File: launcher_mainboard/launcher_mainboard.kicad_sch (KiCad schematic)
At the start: 76 parts, among them J10 header, J11 header, J12 USB_C_Receptacle_USB2.0_16P, J2 Conn_01x06, J3 Conn_01x06, J4 Conn_01x06, J5 Conn_01x06, J6 bat_con, J7 fan_con, J8 ESC_1, J9 ESC_2, Q1 PJC7400, Q4 BSS138, Q5 BSS138, Q6 BSS138, Q7 BSS138, SW1 POWER_SWITCH, U1 R-78E3.3-1.0, U10 TLV75533PDBV, U12 LM66200DRLR, U2 TMC2209-LA-T, U3 TMC2209-LA-T, U4 TMC2209-LA-T, U5 TMC2209-LA-T, U6 ESP32-S3-WROOM-1, U8 D3V3XA4B10LP, U9 R-78E5.0-0.5

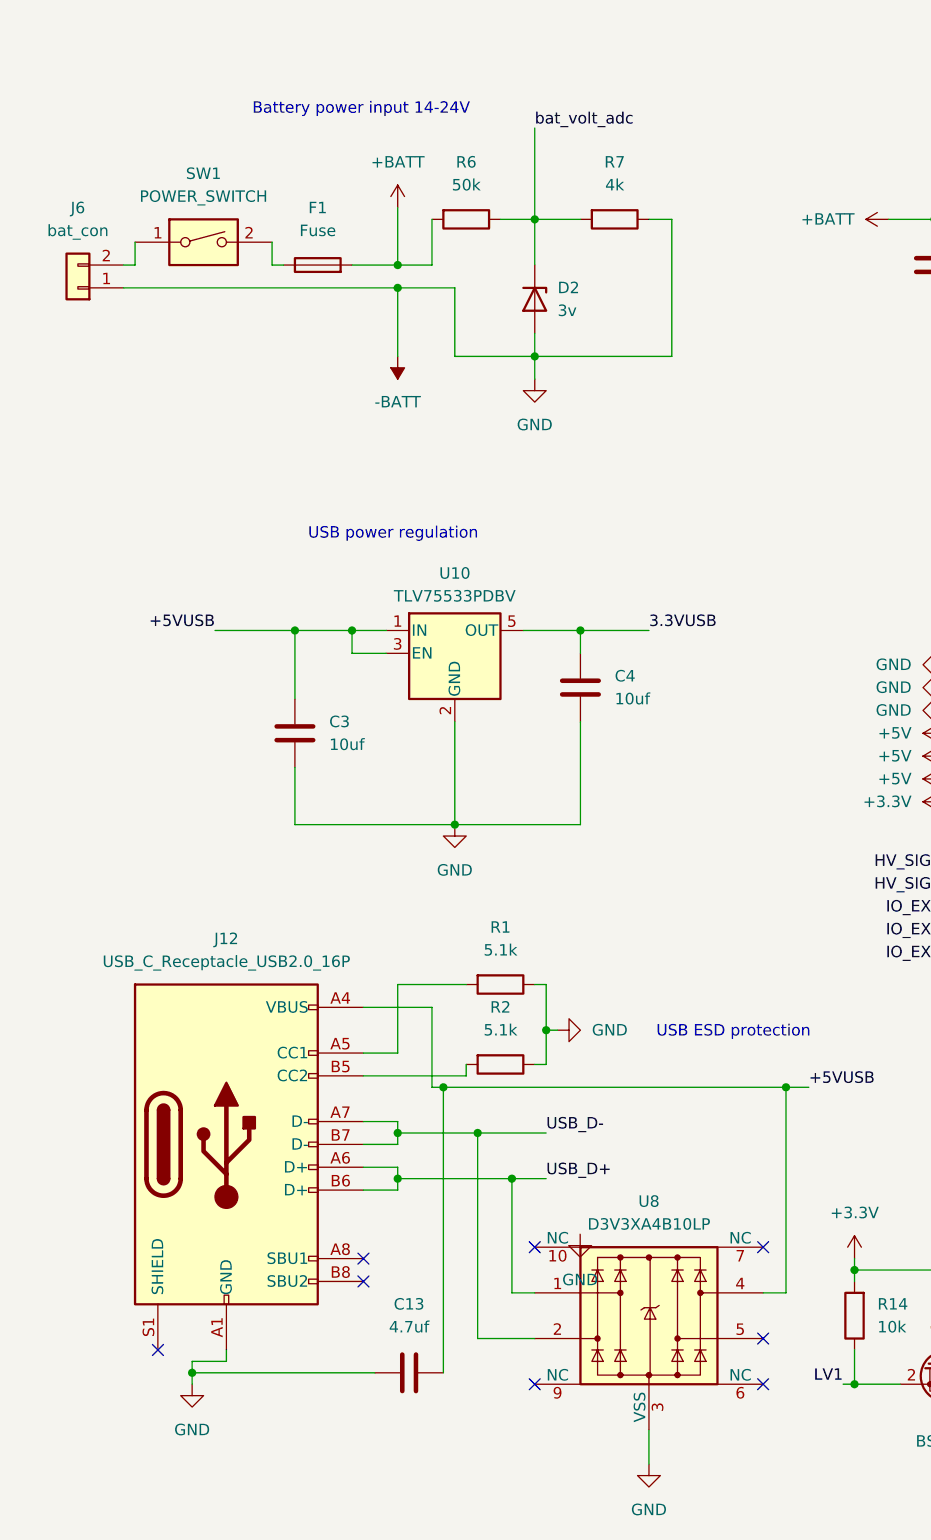
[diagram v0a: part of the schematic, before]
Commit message: project restructure, switched out EDC IC, more layout
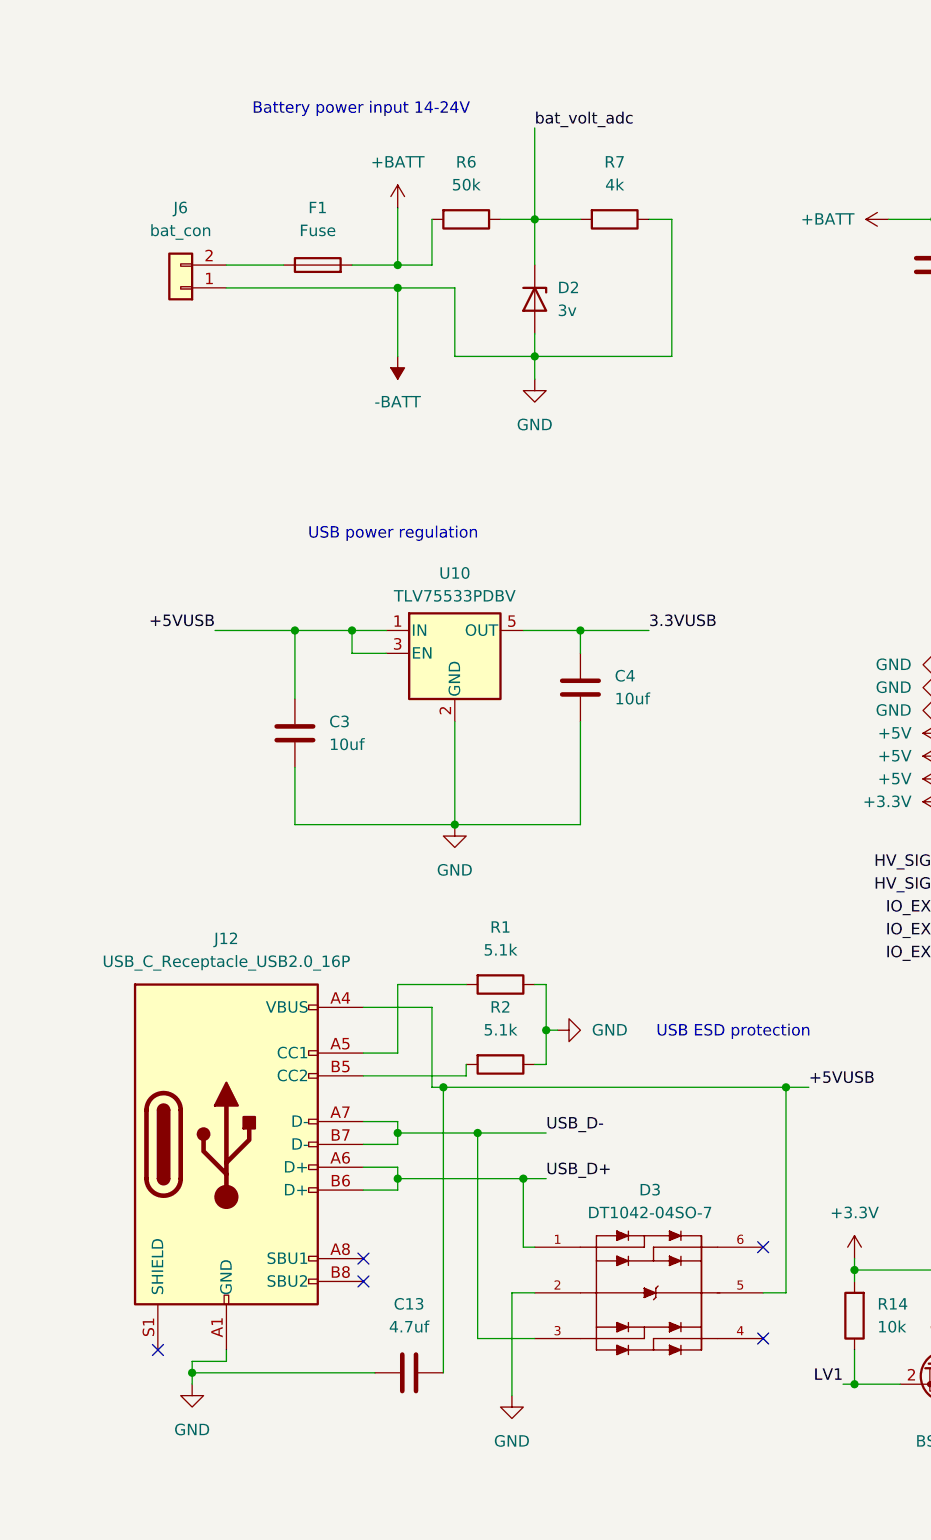
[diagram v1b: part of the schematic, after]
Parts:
- removed SW1: POWER_SWITCH, Button_Switch_SMD:SW_DIP_SPSTx01_Slide_9.78x4.72mm_W8.61mm_P2.54mm, symbol Switch:SW_DIP_x01
- removed U8: D3V3XA4B10LP, Package_DFN_QFN:Diodes_UDFN-10_1.0x2.5mm_P0.5mm, symbol Power_Protection:D3V3XA4B10LP
- added D3: DT1042-04SO-7, DT1042:SOT95P285X140-6N, symbol DT1042:DT1042-04SO-7
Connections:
- net +5VUSB: now also D3.5
- net -BATT: now also D3.2
- net USB_D+: now also D3.1
- net USB_D-: now also D3.3
- net at J6.2 (Pin_2): now also F1.1
- no-connect marks 59 -> 56
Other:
- moved on the sheet: J6
